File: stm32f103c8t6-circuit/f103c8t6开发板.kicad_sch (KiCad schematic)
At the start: 0 parts

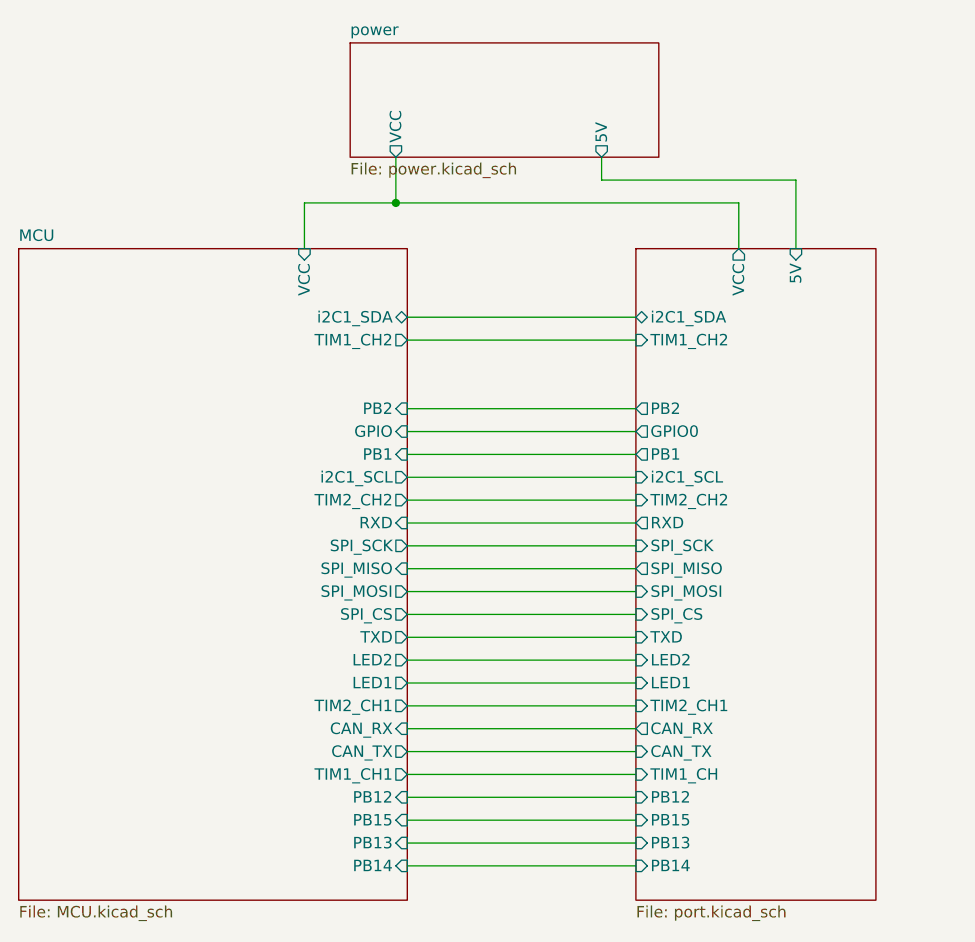
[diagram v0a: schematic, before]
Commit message: Modify PCH and SCH
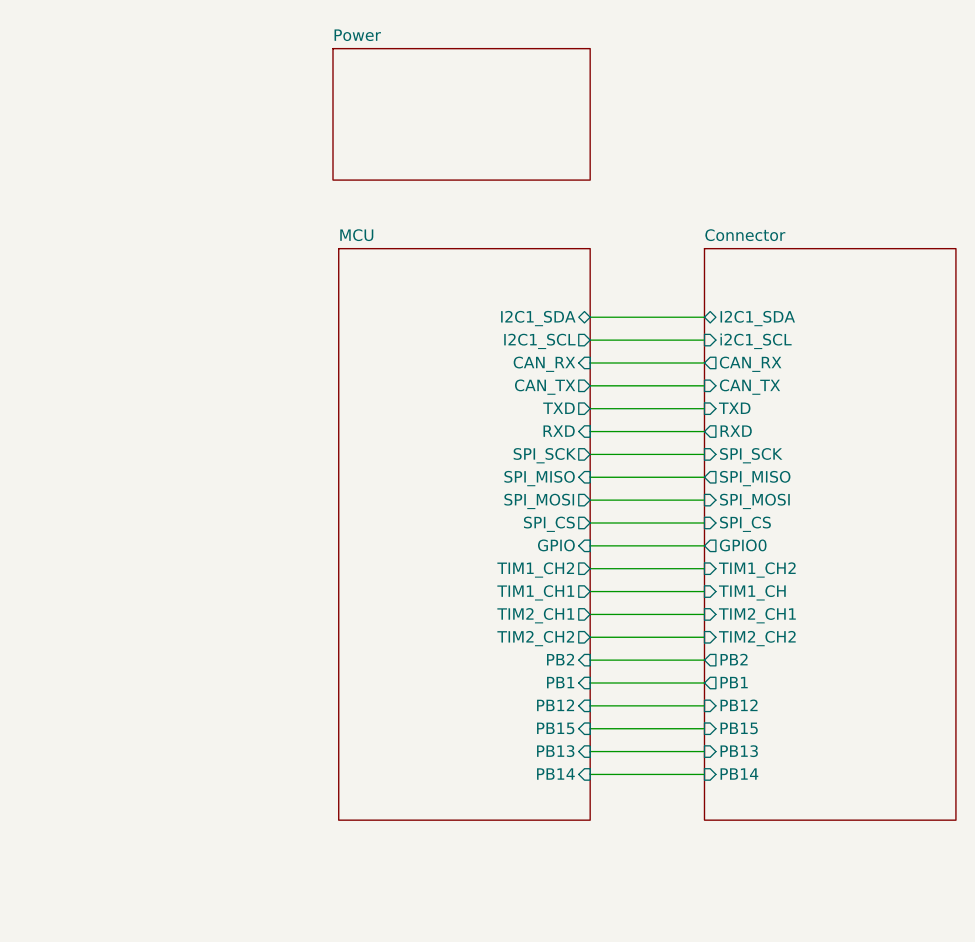
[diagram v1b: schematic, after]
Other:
- sheet port renamed Connector
- sheet power renamed Power
- sheet Connector ports: added I2C1_SDA; removed 5V, LED1, LED2, VCC, i2C1_SDA
- sheet MCU ports: added I2C1_SCL, I2C1_SDA; removed LED1, LED2, VCC, i2C1_SCL, i2C1_SDA
- sheet Power ports: added none; removed 5V, VCC
